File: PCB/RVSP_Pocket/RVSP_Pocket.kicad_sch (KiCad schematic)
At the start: 1 part, among them U1 STM32F401CCUx

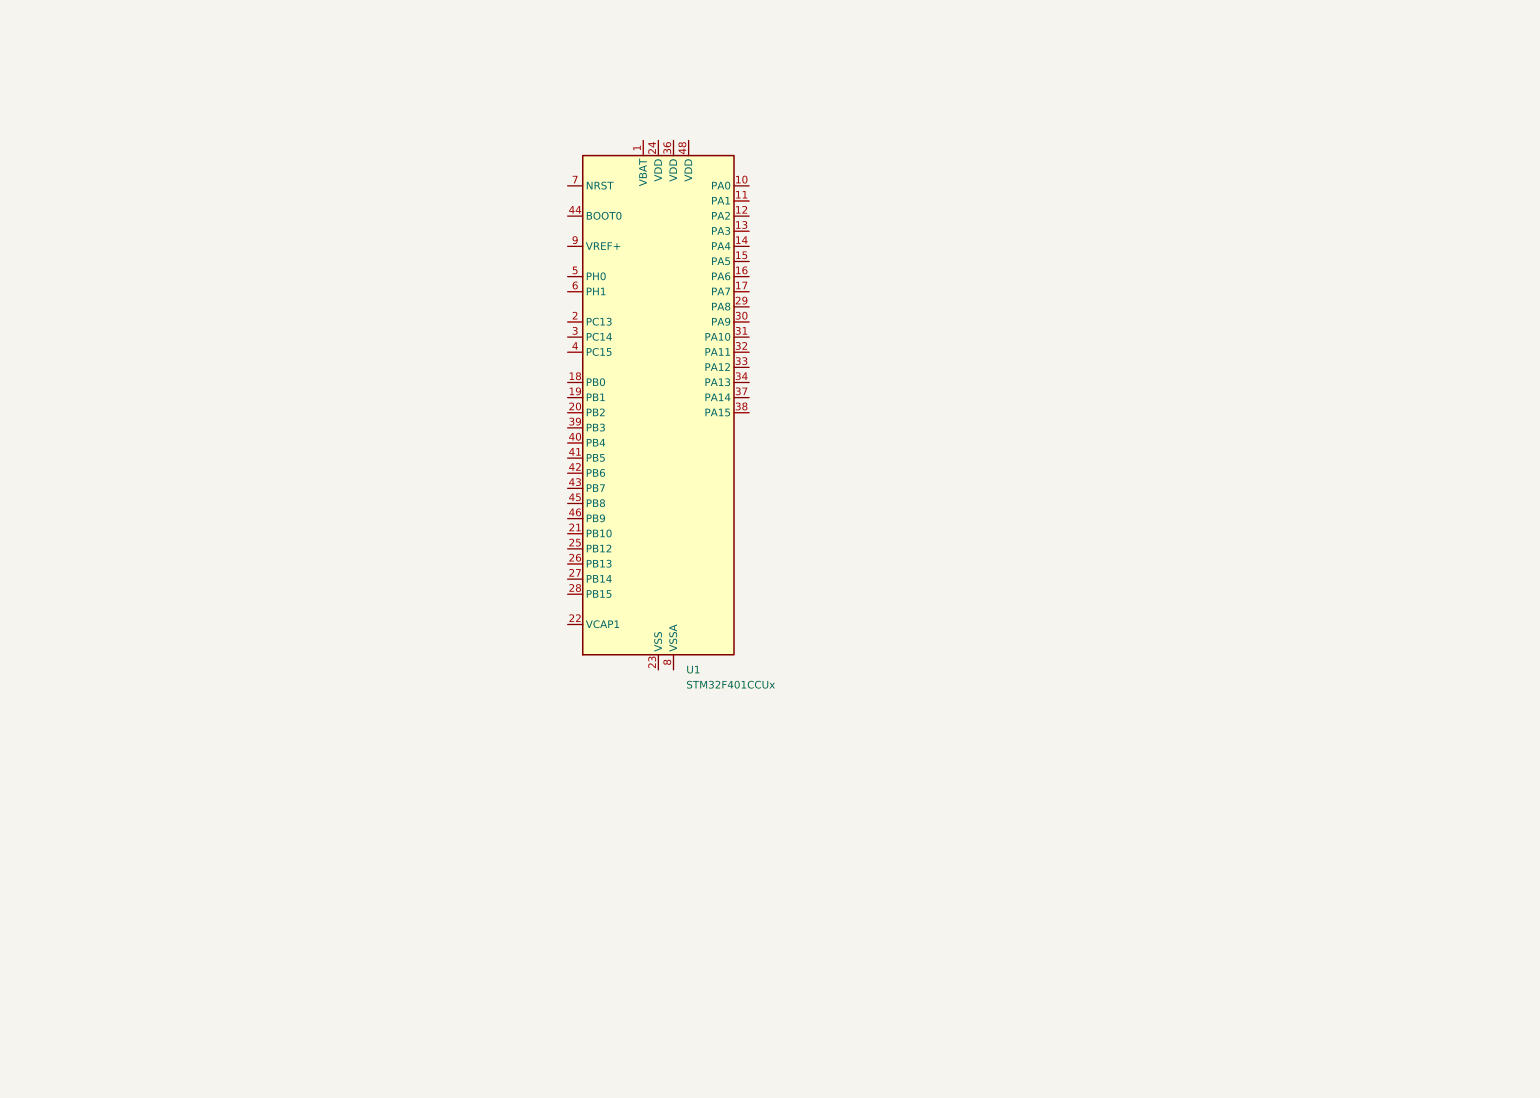
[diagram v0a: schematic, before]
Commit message: Added PCB files
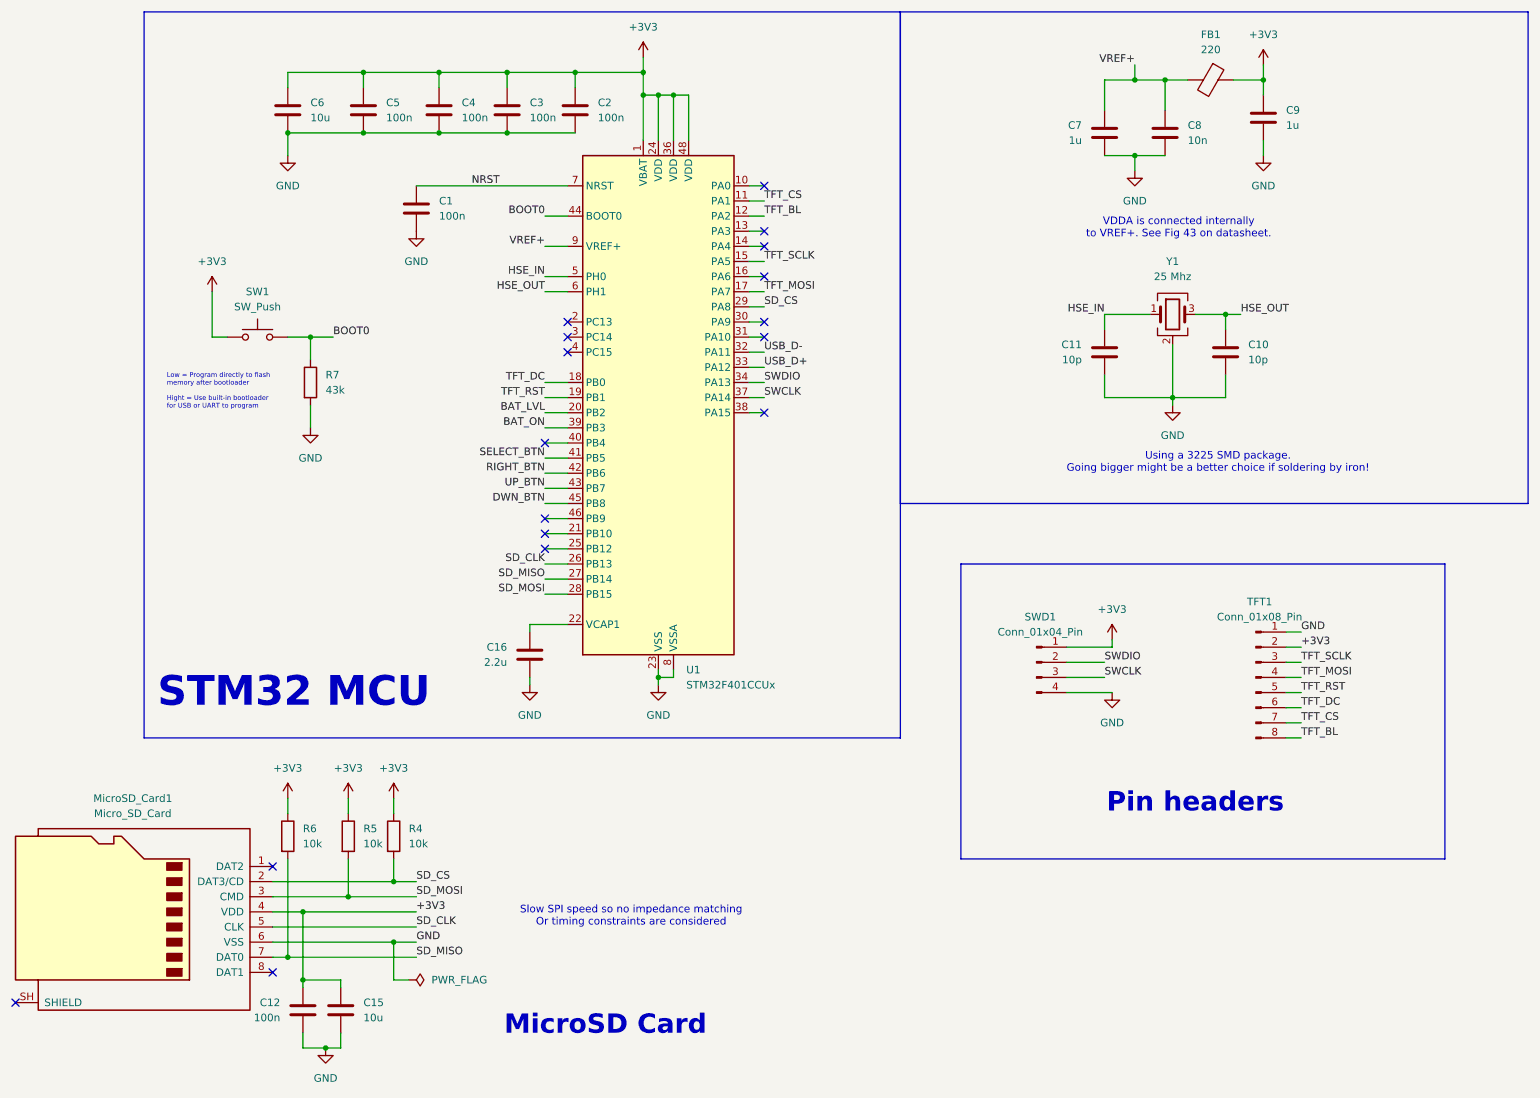
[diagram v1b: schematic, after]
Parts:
- added C1, C12, C2, C3, C4, C5: 100n, Capacitor_SMD:C_0603_1608Metric_Pad1.08x0.95mm_HandSolder, symbol Device:C
- added C10, C11: 10p, Capacitor_SMD:C_0603_1608Metric_Pad1.08x0.95mm_HandSolder, symbol Device:C
- added C15, C6: 10u, Capacitor_SMD:C_0603_1608Metric_Pad1.08x0.95mm_HandSolder, symbol Device:C
- added C16: 2.2u, Capacitor_SMD:C_0603_1608Metric_Pad1.08x0.95mm_HandSolder, symbol Device:C
- added C7, C9: 1u, Capacitor_SMD:C_0603_1608Metric_Pad1.08x0.95mm_HandSolder, symbol Device:C
- added C8: 10n, Capacitor_SMD:C_0603_1608Metric_Pad1.08x0.95mm_HandSolder, symbol Device:C
- added FB1: 220, Resistor_SMD:R_1206_3216Metric_Pad1.30x1.75mm_HandSolder, symbol Device:FerriteBead
- added MicroSD_Card1: Micro_SD_Card, EasyEDA:TF-SMD_XKTF-N02-N, symbol Connector:Micro_SD_Card
- added R4, R5, R6: 10k, Resistor_SMD:R_0603_1608Metric_Pad0.98x0.95mm_HandSolder, symbol Device:R
- added R7: 43k, Resistor_SMD:R_0603_1608Metric_Pad0.98x0.95mm_HandSolder, symbol Device:R
- added SW1: SW_Push, Button_Switch_SMD:SW_SPST_PTS647_Sx38, symbol Switch:SW_Push
- added SWD1: Conn_01x04_Pin, Connector_PinHeader_2.54mm:PinHeader_1x04_P2.54mm_Vertical, symbol Connector:Conn_01x04_Pin
- added TFT1: Conn_01x08_Pin, Connector_PinHeader_2.54mm:PinHeader_1x08_P2.54mm_Vertical, symbol Connector:Conn_01x08_Pin
- added Y1: 25 Mhz, Crystal:Crystal_SMD_3225-4Pin_3.2x2.5mm_HandSoldering, symbol Device:Crystal_GND24
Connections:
- net +3V3: now reaches U1.1 (VBAT)
- net +3V3: now also U1.24 (VDD), U1.36 (VDD), U1.48 (VDD), C12.1, C15.1, C2.1, C3.1, C4.1, C5.1, C6.1, C9.1, FB1.1, MicroSD_Card1.4 (VDD), R4.1, R5.1, R6.1, SW1.1, SWD1.1 (Pin_1), TFT1.2 (Pin_2)
- net TFT_CS: now reaches U1.11 (PA1)
- net TFT_CS: now also TFT1.7 (Pin_7)
- net TFT_BL: now reaches U1.12 (PA2)
- net TFT_BL: now also TFT1.8 (Pin_8)
- net TFT_SCLK: now reaches U1.15 (PA5)
- net TFT_SCLK: now also TFT1.3 (Pin_3)
- net TFT_MOSI: now reaches U1.17 (PA7)
- net TFT_MOSI: now also TFT1.4 (Pin_4)
- net TFT_DC: now reaches U1.18 (PB0)
- net TFT_DC: now also TFT1.6 (Pin_6)
- net TFT_RST: now reaches U1.19 (PB1)
- net TFT_RST: now also TFT1.5 (Pin_5)
- net BAT_LVL: now reaches U1.20 (PB2)
- net at U1.22 (VCAP1): now also C16.1
- net GND: now reaches U1.23 (VSS), U1.35 (VSS), U1.47 (VSS), U1.49 (VSS)
- net GND: now also U1.8 (VSSA), C1.2, C10.2, C11.2, C12.2, C15.2, C16.2, C2.2, C3.2, C4.2, C5.2, C6.2, C7.2, C8.2, C9.2, MicroSD_Card1.6 (VSS), R7.2, SWD1.4 (Pin_4), TFT1.1 (Pin_1), Y1.2 (G), Y1.4 (G)
- net SD_CLK: now reaches U1.26 (PB13)
- net SD_CLK: now also MicroSD_Card1.5 (CLK)
- net SD_MISO: now reaches U1.27 (PB14)
- net SD_MISO: now also MicroSD_Card1.7 (DAT0), R6.2
- net SD_MOSI: now reaches U1.28 (PB15)
- net SD_MOSI: now also MicroSD_Card1.3 (CMD), R5.2
- net SD_CS: now reaches U1.29 (PA8)
- net SD_CS: now also MicroSD_Card1.2 (DAT3/CD), R4.2
- net USB_D-: now reaches U1.32 (PA11)
- net USB_D+: now reaches U1.33 (PA12)
- net SWDIO: now reaches U1.34 (PA13)
- net SWDIO: now also SWD1.2 (Pin_2)
- net SWCLK: now reaches U1.37 (PA14)
- net SWCLK: now also SWD1.3 (Pin_3)
- net BAT_ON: now reaches U1.39 (PB3)
- net SELECT_BTN: now reaches U1.41 (PB5)
- net RIGHT_BTN: now reaches U1.42 (PB6)
- net UP_BTN: now reaches U1.43 (PB7)
- net BOOT0: now reaches U1.44 (BOOT0)
- net BOOT0: now also R7.1, SW1.2
- net DWN_BTN: now reaches U1.45 (PB8)
- net HSE_IN: now reaches U1.5 (PH0)
- net HSE_IN: now also C11.1, Y1.1
- net HSE_OUT: now reaches U1.6 (PH1)
- net HSE_OUT: now also C10.1, Y1.3
- net NRST: now reaches U1.7 (NRST)
- net NRST: now also C1.1
- net VREF+: now reaches U1.9 (VREF+)
- net VREF+: now also C7.1, C8.1, FB1.2
- no-connect marks 0 -> 17
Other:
- note added: "Low = Program directly to flash memory after bootloader Hight = Use built-in bootloader for USB or UART to program"
- note added: "MicroSD Card"
- note added: "Pin headers"
- note added: "STM32 MCU"
- note added: "Slow SPI speed so no impedance matching Or timing constraints are considered"
- note added: "Using a 3225 SMD package. Going bigger might be a better choice if soldering by iron!"
- note added: "VDDA is connected internally to VREF+. See Fig 43 on datasheet."
